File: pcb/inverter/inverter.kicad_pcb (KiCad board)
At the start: 2 copper layers, 100 x 61.5 mm, 52 parts, among them J1 Conn_01x01_Female, J1001 mounting-hole-nc, J1002 mounting-hole-nc, J1003 mounting-hole-nc, J1004 mounting-hole-nc, J1005 mounting-hole-grounded, J1006 mounting-hole-grounded, J1007 mounting-hole-grounded, J1008 mounting-hole-grounded, J2 Conn_01x01_Female, J3 Conn_01x01_Female, J4 Conn_01x01_Female, J5 Conn_01x02_Male, J6 Conn_01x02_Male, J7 Conn_01x02_Male, J8 Conn_01x02_Male, Q1 IRG4PF50W, Q2 IRG4PF50W, Q3 IRG4PF50W, Q4 IRG4PF50W, Q5 IRG4PF50W, Q6 IRG4PF50W, Q7 IRG4PF50W, Q8 IRG4PF50W

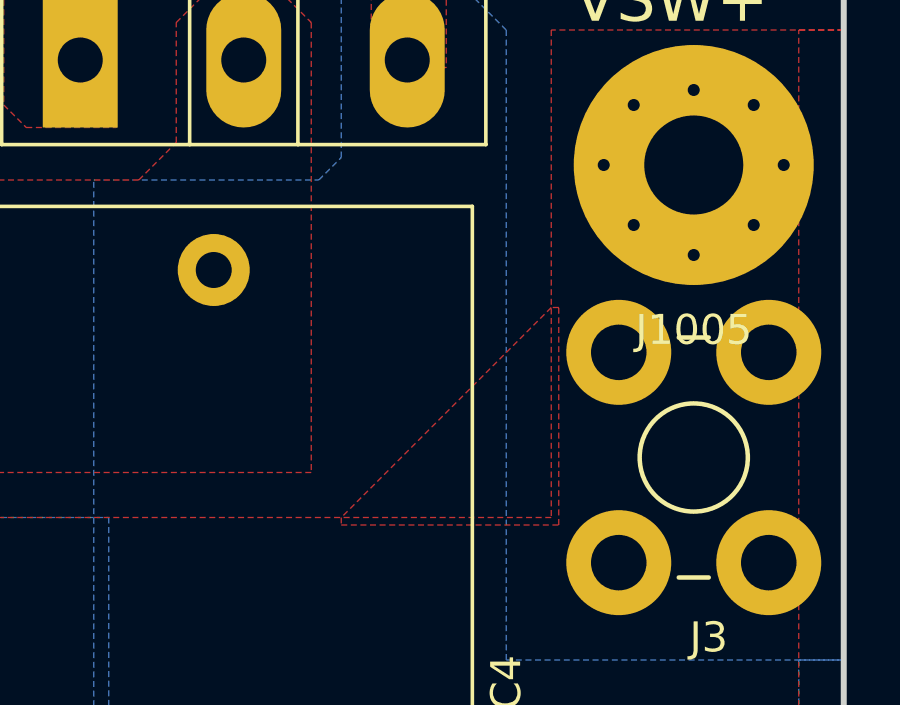
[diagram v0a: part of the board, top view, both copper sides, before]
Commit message: regenerated all gerbers and ordered controller and inverter pcbs
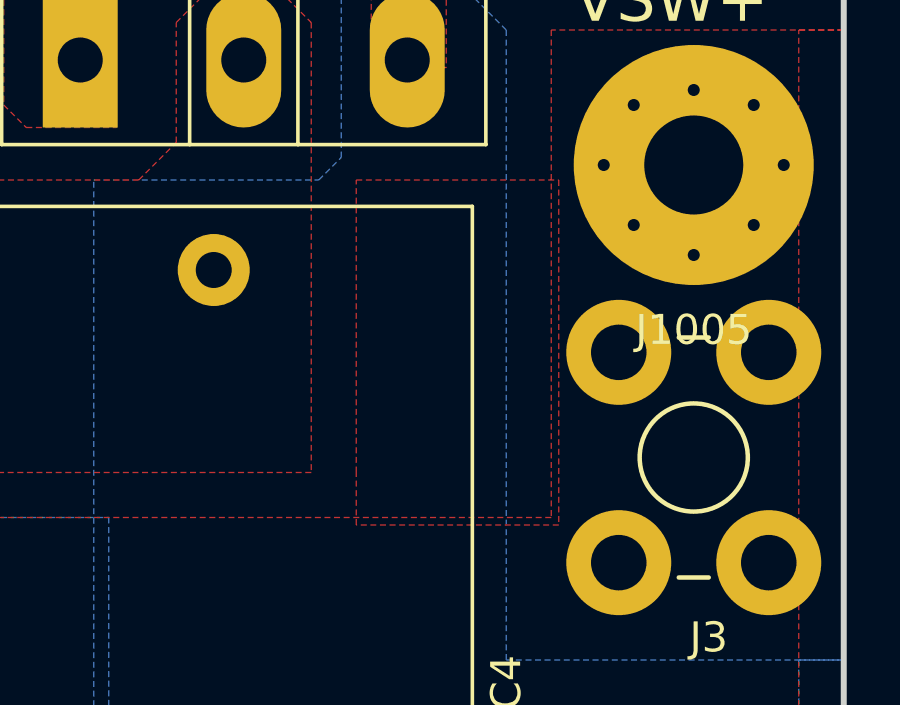
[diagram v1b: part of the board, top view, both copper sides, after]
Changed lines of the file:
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@@
-(kicad_pcb (version 20171130) (host pcbnew "(5.0.1-3-g963ef8bb5)")
+(kicad_pcb (version 20171130) (host pcbnew 5.0.2-bee76a0~70~ubuntu18.04.1)
   (general
     (thickness 1.6)
@@
   )
   (zone (net 6) (net_name /VSW+) (layer F.Cu) (hatch edge 0.508)
-    (connect_pads yes (clearance 1))
-    (min_thickness 0.254)
-    (fill yes (arc_segments 16) (thermal_gap 0.508) (thermal_bridge_width 0.508))
-    (polygon
-      (pts
-        (xy 191 63.25) (xy 190.75 63.25) (xy 183.75 70.25) (xy 183.75 70.5) (xy 191 70.5)
-      )
-    )
-  )
-  (zone (net 6) (net_name /VSW+) (layer F.Cu) (hatch edge 0.508)
     (connect_pads yes (clearance 0.25))
     (min_thickness 0.2)
@@
       )
     )
+  )
+  (zone (net 0) (net_name "") (layer B.Cu) (hatch edge 0.508)
+    (connect_pads (clearance 0.49))
+    (min_thickness 0.254)
+    (keepout (tracks allowed) (vias allowed) (copperpour not_allowed))
+    (fill (arc_segments 16) (thermal_gap 0.508) (thermal_bridge_width 0.508))
+    (polygon
+      (pts
+        (xy 190.25 93.5) (xy 190.25 89.5) (xy 189.25 89.5) (xy 189.25 93.5)
+      )
+    )
+  )
+  (zone (net 6) (net_name /VSW+) (layer F.Cu) (hatch edge 0.508)
+    (connect_pads yes (clearance 0.49))
+    (min_thickness 0.254)
+    (fill yes (arc_segments 16) (thermal_gap 0.508) (thermal_bridge_width 0.508))
+    (polygon
+      (pts
+        (xy 184.25 68.75) (xy 184.25 59) (xy 191 59) (xy 191 70.5) (xy 184.25 70.5)
+      )
+    )
